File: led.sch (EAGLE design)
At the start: 44 parts, among them U1 TPS92513HV, U2 TPS92513HV

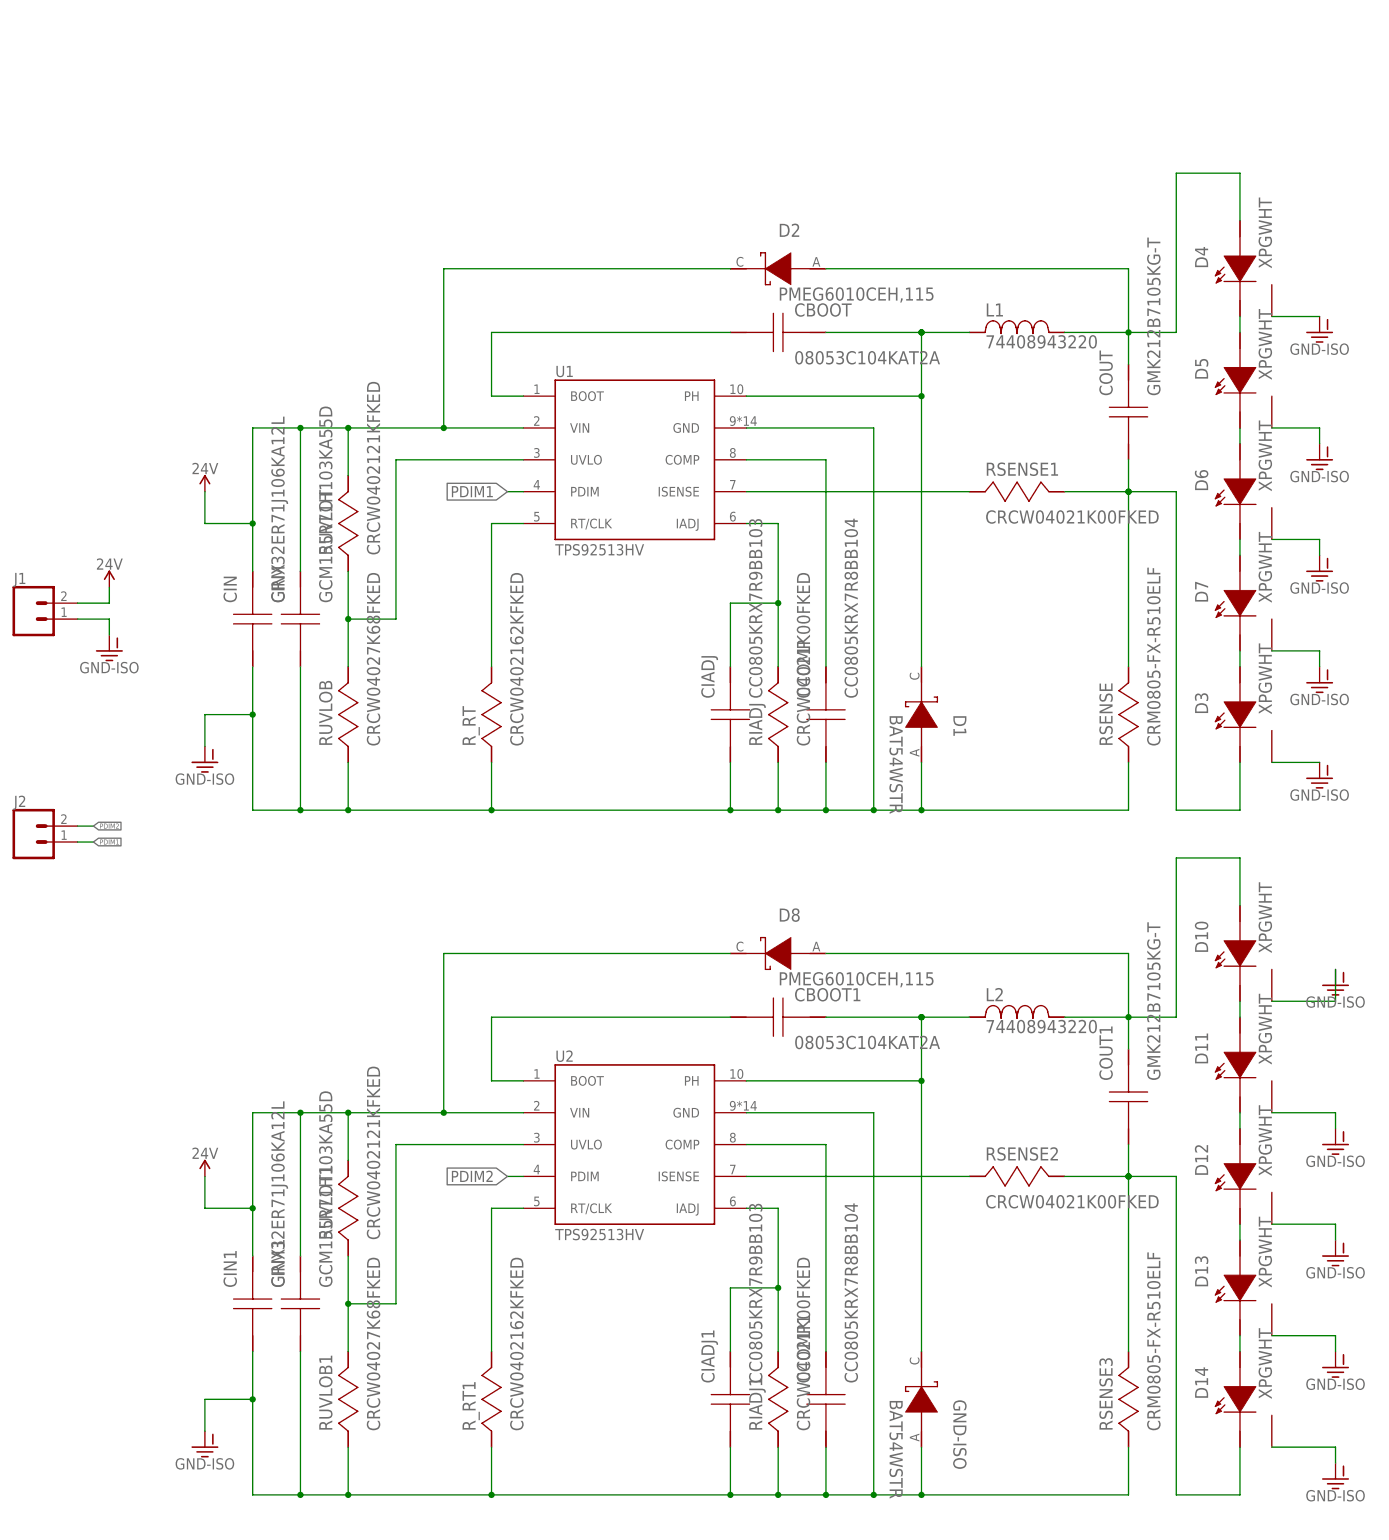
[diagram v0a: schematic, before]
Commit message: should be good to order parts
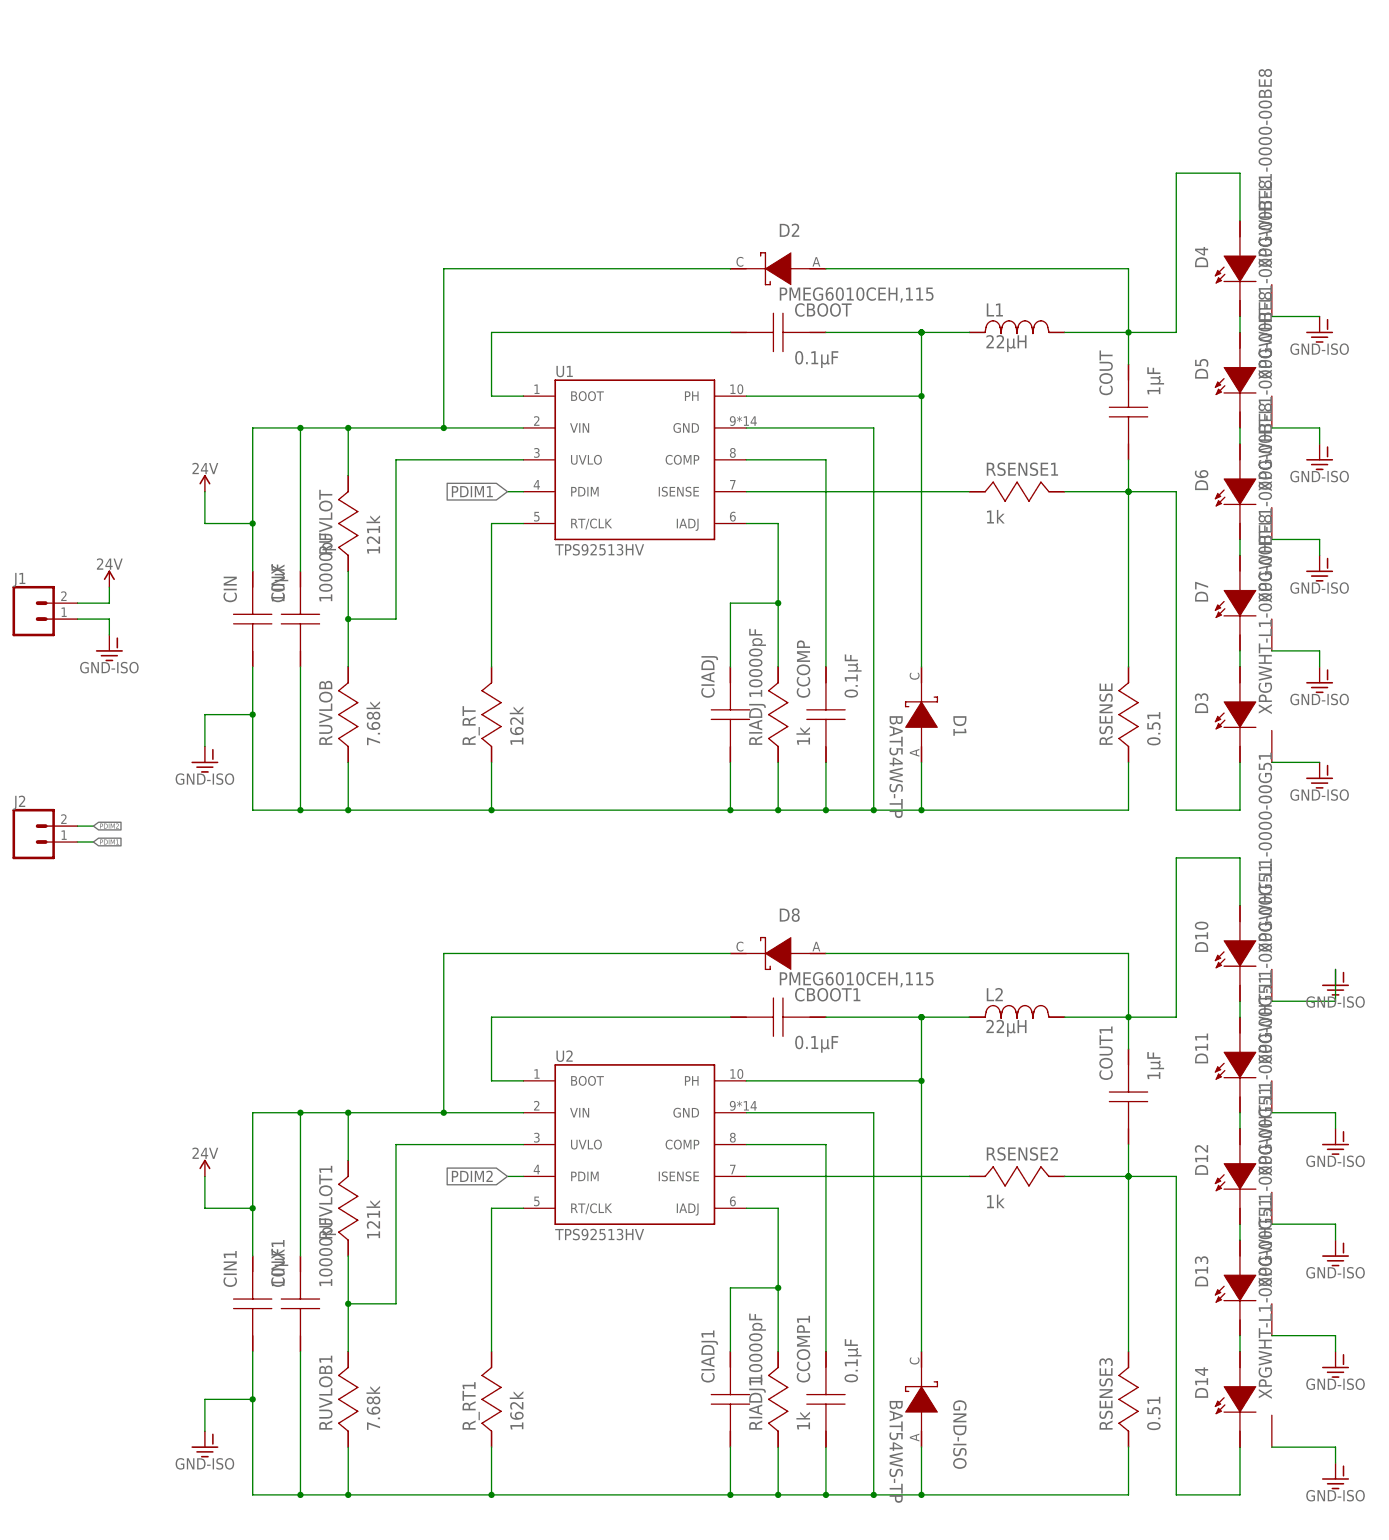
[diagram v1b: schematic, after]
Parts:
- CBOOT, CBOOT1: value 08053C104KAT2A -> 0.1µF
- CCOMP, CCOMP1: value CC0805KRX7R8BB104 -> 0.1µF
- CIADJ, CIADJ1: value CC0805KRX7R9BB103 -> 10000pF
- CIN, CIN1: value GRM32ER71J106KA12L -> 10µF; device derek:GRM32ER71J106KA12L -> derek:GRM32ER71J106MA12L
- CINX, CINX1: value GCM155R71H103KA55D -> 10000pF
- COUT, COUT1: value GMK212B7105KG-T -> 1µF
- D1, GND-ISO: value BAT54WSTR -> BAT54WS-TP; device derek:BAT54WSTR -> derek:BAT54WS-TP
- D10, D11, D12, D13, D14: value XPGWHT -> XPGWHT-L1-0000-00G51; device derek:XPGWHT -> derek:XPGWHT-L1-0000-00G51
- D3, D4, D5, D6, D7: value XPGWHT -> XPGWHT-L1-0000-00BE8; device derek:XPGWHT -> derek:XPGWHT-L1-0000-00BE8
- L1, L2: value 74408943220 -> 22µH
- RIADJ, RIADJ1, RSENSE1, RSENSE2: value CRCW04021K00FKED -> 1k; device derek:CRCW04021K00FKED -> derek:CRCW04021K00DHEDP
- RSENSE, RSENSE3: value CRM0805-FX-R510ELF -> 0.51
- RUVLOB, RUVLOB1: value CRCW04027K68FKED -> 7.68k
- RUVLOT, RUVLOT1: value CRCW0402121KFKED -> 121k
- R_RT, R_RT1: value CRCW0402162KFKED -> 162k
